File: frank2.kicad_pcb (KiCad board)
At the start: 2 copper layers, 77.3 x 99 mm, 150 parts, among them J1 USB Data, J2 Keyboard Data, Q1 BC850, Q2 BC850, SW1 Flash Button, SW2 Reset Button, SW3 Flash Button, U1 NCP1117-3.3_SOT223, U2 RP2040, Y1 ABM8-272-T3, Y2 ABM8-272-T3

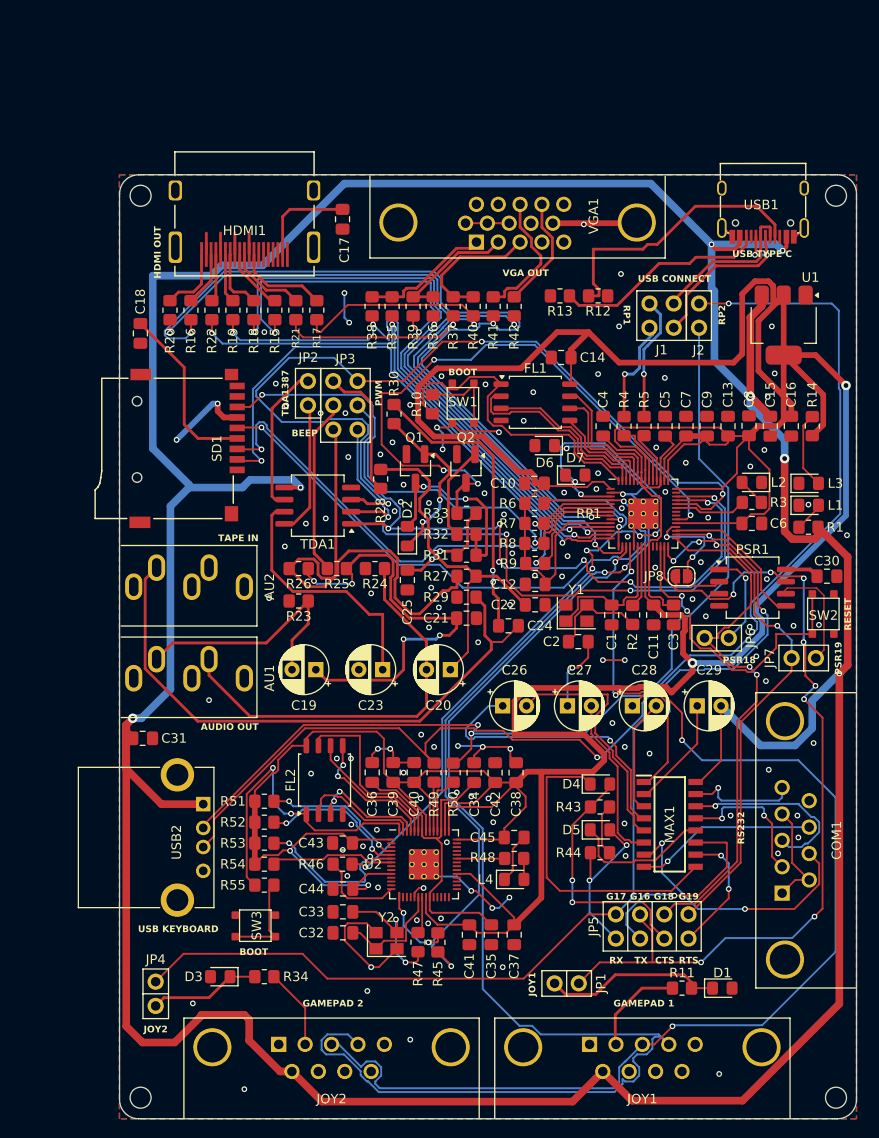
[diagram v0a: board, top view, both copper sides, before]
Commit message: Updated HW
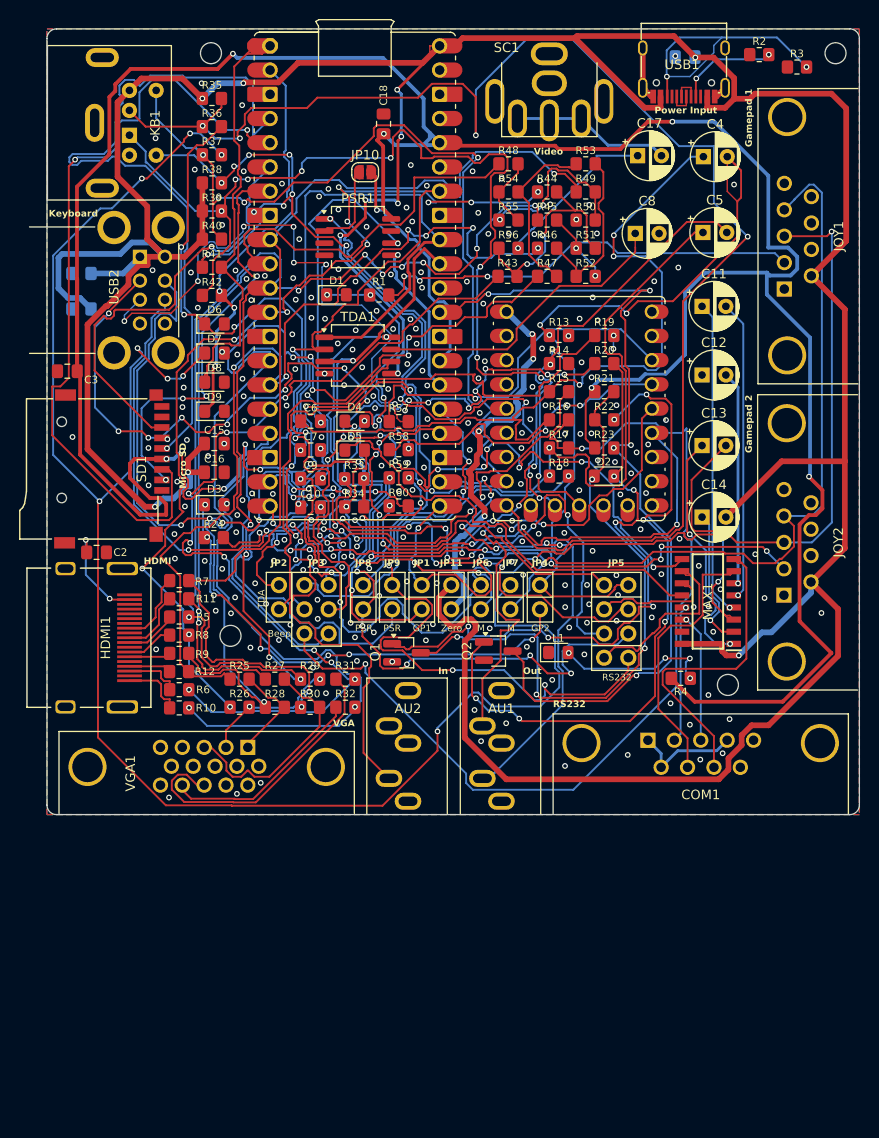
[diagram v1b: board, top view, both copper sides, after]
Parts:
- removed C21, C22: 10n, Capacitor_SMD:C_0805_2012Metric_Pad1.18x1.45mm_HandSolder
- removed C23: 10u, LIBS:Medved_CP_Radial_D5.0mm_P2.50mm
- removed C24, C25, C30: 0.1u, Capacitor_SMD:C_0805_2012Metric_Pad1.18x1.45mm_HandSolder
- removed C26, C27, C28, C29: 1u, LIBS:Medved_CP_Radial_D5.0mm_P2.50mm
- removed C31: 10u, Capacitor_SMD:C_0805_2012Metric_Pad1.18x1.45mm_HandSolder
- removed C32, C33: 15p, Capacitor_SMD:C_0805_2012Metric_Pad1.18x1.45mm_HandSolder
- removed C34, C35, C37, C39, C40, C41, C42, C43, C44, C45: 100n, Capacitor_SMD:C_0805_2012Metric_Pad1.18x1.45mm_HandSolder
- removed C36, C38: 1u, Capacitor_SMD:C_0805_2012Metric_Pad1.18x1.45mm_HandSolder
- removed FL1, FL2: W25Q128JVS, Package_SO:SOIC-8_5.23x5.23mm_P1.27mm
- removed J1: USB Data, LIBS:Medved_2x02
- removed J2: Keyboard Data, LIBS:Medved_PinHeader_1x02
- removed L2, L3, L4: LED, LED_SMD:LED_0805_2012Metric_Pad1.15x1.40mm_HandSolder
- removed REF** (x4): Medved_MountingHole_V2, LIBS:Medved_MountingHole_V2
- removed SW1, SW3: Flash Button, LIBS:Button_SMD_3x3x2
- removed SW2: Reset Button, LIBS:Button_SMD_3x3x2
- removed U1: NCP1117-3.3_SOT223, Package_TO_SOT_SMD:SOT-223-3_TabPin2
- removed U2: RP2040, LIBS:RP2040-QFN-56
- removed Y1, Y2: ABM8-272-T3, Crystal:Crystal_SMD_3225-4Pin_3.2x2.5mm
- added D8: 3V3, LIBS:Medved_D_0805, F.Cu at (94.8, 64.9)
- added D9: 3V3, LIBS:Medved_D_0805, F.Cu at (94.8, 67.9)
- added H1: MountingHole, LIBS:Medved_MountingHole_V2, F.Cu at (94.4, 30.4)
- added H2: MountingHole, LIBS:Medved_MountingHole_V2, F.Cu at (159.9, 30.4)
- added H3: MountingHole, LIBS:Medved_MountingHole_V2, F.Cu at (148.6, 96.6)
- added H4: MountingHole, LIBS:Medved_MountingHole_V2, F.Cu at (96.4, 91.5)
- added JP10: JMP PSRAM, Jumper:SolderJumper-2_P1.3mm_Open_RoundedPad1.0x1.5mm, F.Cu at (110.6, 42.8)
- added JP11: RP ZERO +5V Jumper, LIBS:Medved_PinHeader_1x02_P2.54mm_Vertical_R, F.Cu at (119.6, 86.1)
- added JP9: RP ZERO +5V Jumper, LIBS:Medved_PinHeader_1x02_P2.54mm_Vertical_R, F.Cu at (113.4, 86.1)
- added KB1: PS/2, LIBS:Connector_Mini-DIN_Female_6Pin_2rows, F.Cu at (85.8, 39.0)
- added R56: 51R*, LIBS:Medved_R_0805, F.Cu at (125.6, 50.8)
- added R57: 22R, LIBS:Medved_R_0805, F.Cu at (114.1, 69.0)
- added R58: 22R, LIBS:Medved_R_0805, F.Cu at (114.1, 71.9)
- added R59: 22R, LIBS:Medved_R_0805, F.Cu at (114.1, 74.9)
- added R60: 22R, LIBS:Medved_R_0805, F.Cu at (114.1, 77.8)
- added RP2: RP 2040 Zero, LIBS:rp2040-zero-tht, F.Cu at (133.0, 67.6)
- added SC1: VIDEO (Soft Composite), LIBS:AV_MOD_III-8.4-5, F.Cu at (129.9, 34.1)
- C1: value 15p -> 10u; footprint Capacitor_SMD:C_0805_2012Metric_Pad1.18x1.45mm_HandSolder -> LIBS:Medved_C_0805; moved to B.Cu
- C10, C3, C9: value 100n -> 0.1u; footprint Capacitor_SMD:C_0805_2012Metric_Pad1.18x1.45mm_HandSolder -> LIBS:Medved_C_0805
- C11, C12, C13, C14: value 100n -> 1u; footprint Capacitor_SMD:C_0805_2012Metric_Pad1.18x1.45mm_HandSolder -> LIBS:Medved_CP_Radial_D5.0mm_P2.50mm
- C15, C16: value 10u -> 0.1u; footprint Capacitor_SMD:C_0805_2012Metric_Pad1.18x1.45mm_HandSolder -> LIBS:Medved_C_0805
- C17: value 0.1u -> 220u; footprint Capacitor_SMD:C_0805_2012Metric_Pad1.18x1.45mm_HandSolder -> LIBS:Medved_CP_Radial_D5.0mm_P2.50mm
- C18: footprint Capacitor_SMD:C_0805_2012Metric_Pad1.18x1.45mm_HandSolder -> LIBS:Medved_C_0805
- C19, C20: footprint LIBS:Medved_CP_Radial_D5.0mm_P2.50mm -> LIBS:Medved_R_0805; moved to B.Cu
- C2: value 15p -> 0.1u; footprint Capacitor_SMD:C_0805_2012Metric_Pad1.18x1.45mm_HandSolder -> LIBS:Medved_C_0805
- C4, C8: value 100n -> 10u; footprint Capacitor_SMD:C_0805_2012Metric_Pad1.18x1.45mm_HandSolder -> LIBS:Medved_CP_Radial_D5.0mm_P2.50mm
- C5: value 1u -> 10u; footprint Capacitor_SMD:C_0805_2012Metric_Pad1.18x1.45mm_HandSolder -> LIBS:Medved_CP_Radial_D5.0mm_P2.50mm
- C6: value 100n -> 10n; footprint Capacitor_SMD:C_0805_2012Metric_Pad1.18x1.45mm_HandSolder -> LIBS:Medved_C_0805
- C7: value 1u -> 10n; footprint Capacitor_SMD:C_0805_2012Metric_Pad1.18x1.45mm_HandSolder -> LIBS:Medved_C_0805
- D1, D2, D3, D4, D5, D6, D7: footprint Diode_SMD:D_0805_2012Metric_Pad1.15x1.40mm_HandSolder -> LIBS:Medved_D_0805
- JP8: value JMP PSRAM -> RP ZERO +5V Jumper; footprint Jumper:SolderJumper-2_P1.3mm_Open_RoundedPad1.0x1.5mm -> LIBS:Medved_PinHeader_1x02_P2.54mm_Vertical_R
- L1: footprint LED_SMD:LED_0805_2012Metric_Pad1.15x1.40mm_HandSolder -> LIBS:Medved_L_0805
- R1: value 10K -> 1k; footprint Resistor_SMD:R_0805_2012Metric_Pad1.20x1.40mm_HandSolder -> LIBS:Medved_R_0805
- R10, R11, R47: value 1k -> 270R; footprint Resistor_SMD:R_0805_2012Metric_Pad1.20x1.40mm_HandSolder -> LIBS:Medved_R_0805
- R12: value 5.1K -> 270R; footprint Resistor_SMD:R_0805_2012Metric_Pad1.20x1.40mm_HandSolder -> LIBS:Medved_R_0805
- R13: value 5.1K -> 330R; footprint Resistor_SMD:R_0805_2012Metric_Pad1.20x1.40mm_HandSolder -> LIBS:Medved_R_0805
- R14: value 1K -> 330R; footprint Resistor_SMD:R_0805_2012Metric_Pad1.20x1.40mm_HandSolder -> LIBS:Medved_R_0805
- R15, R18: value 270R -> 1k; footprint Resistor_SMD:R_0805_2012Metric_Pad1.20x1.40mm_HandSolder -> LIBS:Medved_R_0805
- R16, R17: value 270R -> 2k; footprint Resistor_SMD:R_0805_2012Metric_Pad1.20x1.40mm_HandSolder -> LIBS:Medved_R_0805
- R19: value 270R -> 100R; footprint Resistor_SMD:R_0805_2012Metric_Pad1.20x1.40mm_HandSolder -> LIBS:Medved_R_0805
- R2: value 1k -> 5.1K; footprint Resistor_SMD:R_0805_2012Metric_Pad1.20x1.40mm_HandSolder -> LIBS:Medved_R_0805
- R20, R21, R22: value 270R -> 10k; footprint Resistor_SMD:R_0805_2012Metric_Pad1.20x1.40mm_HandSolder -> LIBS:Medved_R_0805
- R23, R24, R35: value 330R -> 1k; footprint Resistor_SMD:R_0805_2012Metric_Pad1.20x1.40mm_HandSolder -> LIBS:Medved_R_0805
- R25: value 1k -> 330R; footprint Resistor_SMD:R_0805_2012Metric_Pad1.20x1.40mm_HandSolder -> LIBS:Medved_R_0805
- R26, R27: value 2k -> 330R; footprint Resistor_SMD:R_0805_2012Metric_Pad1.20x1.40mm_HandSolder -> LIBS:Medved_R_0805
- R28, R38, R39, R40, R41, R42: footprint Resistor_SMD:R_0805_2012Metric_Pad1.20x1.40mm_HandSolder -> LIBS:Medved_R_0805
- R29: value 100R -> 1k; footprint Resistor_SMD:R_0805_2012Metric_Pad1.20x1.40mm_HandSolder -> LIBS:Medved_R_0805
- R3: value 1K -> 5.1K; footprint Resistor_SMD:R_0805_2012Metric_Pad1.20x1.40mm_HandSolder -> LIBS:Medved_R_0805
- R30: value 10k -> 1k; footprint Resistor_SMD:R_0805_2012Metric_Pad1.20x1.40mm_HandSolder -> LIBS:Medved_R_0805
- R31, R32: value 10k -> 100R; footprint Resistor_SMD:R_0805_2012Metric_Pad1.20x1.40mm_HandSolder -> LIBS:Medved_R_0805
- R33, R34: value 1k -> 1K; footprint Resistor_SMD:R_0805_2012Metric_Pad1.20x1.40mm_HandSolder -> LIBS:Medved_R_0805
- R36, R37: value 330R -> 100R; footprint Resistor_SMD:R_0805_2012Metric_Pad1.20x1.40mm_HandSolder -> LIBS:Medved_R_0805
- R4: value 27 -> 1K; footprint Resistor_SMD:R_0805_2012Metric_Pad1.20x1.40mm_HandSolder -> LIBS:Medved_R_0805
- R43: value 1K -> 750R*; footprint Resistor_SMD:R_0805_2012Metric_Pad1.20x1.40mm_HandSolder -> LIBS:Medved_R_0805
- R44, R48: value 1K -> 270R; footprint Resistor_SMD:R_0805_2012Metric_Pad1.20x1.40mm_HandSolder -> LIBS:Medved_R_0805
- R45, R46: value 100R -> 270R; footprint Resistor_SMD:R_0805_2012Metric_Pad1.20x1.40mm_HandSolder -> LIBS:Medved_R_0805
- R49, R5: value 27 -> 270R; footprint Resistor_SMD:R_0805_2012Metric_Pad1.20x1.40mm_HandSolder -> LIBS:Medved_R_0805
- R50: value 27 -> 300R; footprint Resistor_SMD:R_0805_2012Metric_Pad1.20x1.40mm_HandSolder -> LIBS:Medved_R_0805
- R51, R52, R53, R54: value 10K -> 150R; footprint Resistor_SMD:R_0805_2012Metric_Pad1.20x1.40mm_HandSolder -> LIBS:Medved_R_0805
- R55: value 1k -> 150R; footprint Resistor_SMD:R_0805_2012Metric_Pad1.20x1.40mm_HandSolder -> LIBS:Medved_R_0805
- R6, R7, R8, R9: value 10K -> 270R; footprint Resistor_SMD:R_0805_2012Metric_Pad1.20x1.40mm_HandSolder -> LIBS:Medved_R_0805
- RP1: value RP2040 -> RP2040 Pico; footprint LIBS:RP2040-QFN-56 -> LIBS:Raspberry_Pi_Pico_SMT_THT_MOD_2
- USB2: value USB_A -> USB_A_Stacked; footprint LIBS:Medved_USB_A -> LIBS:Medved_USB_A_CUI_UJ2-ADH-TH_Horizontal_Stacked
- moved D1 83.2 mm to (107.6, 55.7)
- moved JOY1 81.8 mm to (154.5, 55.1), turned to 90 degrees
- moved R53 78.8 mm to (133.7, 42.0), turned to 0 degrees
- moved R45 76.6 mm to (129.7, 47.9), turned to 0 degrees
- moved R54 75.0 mm to (125.6, 44.9), turned to 0 degrees
- moved R55 74.3 mm to (125.6, 47.9)
- moved R48 72.9 mm to (125.6, 42.0), turned to 0 degrees
- moved R47 71.1 mm to (129.7, 53.8), turned to 0 degrees
- moved JOY2 70.9 mm to (154.5, 87.2), turned to 90 degrees
- moved R44 69.5 mm to (129.7, 44.9)
- moved C3 68.5 mm to (79.3, 63.7), turned to 0 degrees
- moved R46 68.1 mm to (129.7, 50.8)
- moved R51 67.1 mm to (133.7, 50.8), turned to 0 degrees
- moved R11 66.7 mm to (91.1, 87.6), turned to 0 degrees
- moved R52 66.4 mm to (133.7, 53.8), turned to 0 degrees
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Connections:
- net /PW_D+ renamed /Power/D+
- net /PW_D- renamed /Power/D-
- net /RP2040/GPIO23 renamed /Pico/GPIO29_1
- C1 pad 1: /RP2040/XIN -> VBUS
- C11 pad 1: +3V3 -> /RS232/C2+
- C11 pad 2: GND -> /RS232/C2-
- C12 pad 1: +3V3 -> GND
- C12 pad 2: GND -> /RS232/V-
- C13 pad 1: +3V3 -> /RS232/C1+
- C13 pad 2: GND -> /RS232/C1-
- C14 pad 1: +3V3 -> /RS232/V+
- C14 pad 2: GND -> VBUS
- C16 pad 1: +3V3 -> VBUS
- C17 pad 1: /HDMI/VBUS -> Net-(C17-Pad1)
- C17 pad 2: GND -> /Composite Video/CVBS
- C18 pad 1: GND -> +3V3
- C18 pad 2: /SD/+3V3 -> GND
- C19 pad 1: Net-(C19-Pad1) -> VBUS
- C19 pad 2: /Audio/L -> GND
- C2 pad 1: Net-(C2-Pad1) -> /HDMI/VBUS
- C20 pad 1: Net-(C20-Pad1) -> VBUS
- C20 pad 2: /Audio/R -> GND
- C3 pad 1: Net-(RP1-VREG_VOUT) -> GND
- C3 pad 2: GND -> +3V3
- C4 pad 1: Net-(RP1-VREG_VOUT) -> Net-(C4-Pad1)
- C4 pad 2: GND -> /Audio/L
- C5 pad 1: Net-(RP1-VREG_VOUT) -> Net-(C5-Pad1)
- C5 pad 2: GND -> /Audio/R
- C6 pad 1: +3V3 -> Net-(C4-Pad1)
- C7 pad 1: +3V3 -> Net-(C5-Pad1)
- C8 pad 1: +3V3 -> /Audio/FLT
- C9 pad 1: +3V3 -> /Audio/LOAD_IN
- C9 pad 2: GND -> Net-(C9-Pad2)
- D6 pad 1: /GPIO0 -> Net-(D6-K)
- D7 pad 1: /GPIO1 -> Net-(D7-K)
- JP6 pad 1: Net-(JP6-A) -> /GPIO15
- JP6 pad 2: /GPIO18 -> Net-(D6-K)
- JP7 pad 1: /GPIO19 -> Net-(D7-K)
- JP7 pad 2: Net-(JP7-B) -> /GPIO14
- JP8 pad 2: /GPIO21 -> /GPIO18
- PSR1 pad 1: Net-(JP6-A) -> Net-(JP8-A)
- PSR1 pad 2: Net-(JP8-A) -> Net-(JP10-A)
- PSR1 pad 6: Net-(JP7-B) -> Net-(JP9-B)
- PSR1 pad 8: /PSRAM/+3V3 -> +3V3
- R1 pad 1: Net-(L1-A) -> Net-(D1-K)
- R1 pad 2: VBUS -> /Gamepad 1/J2_DATA
- R10 pad 1: /RP2040/QSPI_SS -> /HDMI/D2P
- R10 pad 2: /RP2040/~{USB_BOOT} -> /GPIO13
- R11 pad 1: Net-(D1-K) -> /HDMI/CLKP
- R11 pad 2: /Gamepad 1/J2_DATA -> /GPIO7
- R12 pad 1: GND -> /HDMI/D1P
- R12 pad 2: Net-(USB1-CC1) -> /GPIO11
- R13 pad 1: GND -> /Audio/L
- R13 pad 2: Net-(USB1-CC2) -> GND
- R14 pad 1: Net-(L3-A) -> /Audio/R
- R14 pad 2: +3V3 -> GND
- R15 pad 1: /HDMI/D0N -> Net-(C4-Pad1)
- R15 pad 2: /GPIO8 -> /Audio/LEFT_OUT
- R16 pad 1: /HDMI/D2N -> Net-(C4-Pad1)
- R16 pad 2: /GPIO12 -> /Audio/BEEP_OUT
- R17 pad 1: /HDMI/CLKN -> Net-(C5-Pad1)
- R17 pad 2: /GPIO6 -> /Audio/BEEP_OUT
- R18 pad 1: /HDMI/D0P -> Net-(C5-Pad1)
- R18 pad 2: /GPIO9 -> /Audio/RIGHT_OUT
- R19 pad 1: /HDMI/D1N -> /Audio/LOAD_IN
- R19 pad 2: /GPIO10 -> GND
- R2 pad 1: /RP2040/XOUT -> GND
- R2 pad 2: Net-(C2-Pad1) -> Net-(USB1-CC1)
- R20 pad 1: /HDMI/D2P -> Net-(C9-Pad2)
- R20 pad 2: /GPIO13 -> Net-(D2-K)
- R21 pad 1: /HDMI/CLKP -> +3V3
- R21 pad 2: /GPIO7 -> Net-(D2-A)
- R22 pad 1: /HDMI/D1P -> Net-(D2-A)
- R22 pad 2: /GPIO11 -> Net-(Q2-B)
- R23 pad 1: /Audio/L -> +3V3
- R23 pad 2: GND -> /GPIO22
- R24 pad 1: /Audio/R -> Net-(D3-K)
- R24 pad 2: GND -> /Gamepad 2/J2_DATA
- R25 pad 1: Net-(C19-Pad1) -> /GPIO11
- R25 pad 2: /Audio/LEFT_OUT -> /VGA/VGA_RH
- R26 pad 1: Net-(C19-Pad1) -> /GPIO9
- R26 pad 2: /Audio/BEEP_OUT -> /VGA/VGA_GH
- R27 pad 1: Net-(C20-Pad1) -> /GPIO7
- R27 pad 2: /Audio/BEEP_OUT -> /VGA/VGA_BH
- R28 pad 1: Net-(C20-Pad1) -> /GPIO10
- R28 pad 2: /Audio/RIGHT_OUT -> /VGA/VGA_RH
- R29 pad 1: /Audio/LOAD_IN -> /GPIO8
- R29 pad 2: GND -> /VGA/VGA_GH
- R3 pad 1: Net-(L2-A) -> GND
- R3 pad 2: /RP2040/GPIO25 -> Net-(USB1-CC2)
- R30 pad 1: Net-(C24-Pad2) -> /GPIO6
- R30 pad 2: Net-(D2-K) -> /VGA/VGA_BH
- R31 pad 1: /Audio/+3V3 -> /VGA/VGA_HS
- R31 pad 2: Net-(D2-A) -> /GPIO12
- R32 pad 1: Net-(D2-A) -> /VGA/VGA_VS
- R32 pad 2: Net-(Q2-B) -> /GPIO13
- R33 pad 1: /Audio/+3V3 -> /RS232/CTS_PICO
- R33 pad 2: /GPIO22 -> +3V3
- R34 pad 1: Net-(D3-K) -> /RS232/RX_PICO
- R34 pad 2: /Gamepad 2/J2_DATA -> +3V3
- R35 pad 1: /GPIO11 -> VBUS
- R35 pad 2: /VGA/VGA_RH -> /ZGPIO14
- R36 pad 1: /GPIO9 -> /ZGPIO14
- R36 pad 2: /VGA/VGA_GH -> Net-(D6-K)
- R37 pad 1: /GPIO7 -> /ZGPIO15
- R37 pad 2: /VGA/VGA_BH -> Net-(D7-K)
- R38 pad 1: /GPIO10 -> VBUS
- R38 pad 2: /VGA/VGA_RH -> /ZGPIO12
- R39 pad 1: /GPIO8 -> VBUS
- R39 pad 2: /VGA/VGA_GH -> /ZGPIO11
- R4 pad 1: /D+ -> Net-(L1-A)
- R4 pad 2: Net-(RP1-USB_DP) -> +3V3
- R40 pad 1: /GPIO6 -> VBUS
- R40 pad 2: /VGA/VGA_BH -> /ZGPIO15
- R41 pad 1: /VGA/VGA_HS -> /ZGPIO12
- R41 pad 2: /GPIO12 -> /GPIO0
- R42 pad 1: /VGA/VGA_VS -> /ZGPIO11
- R42 pad 2: /GPIO13 -> /GPIO1
- R43 pad 1: /RS232/CTS_PICO -> /GPIO12
- R43 pad 2: /RS232/+3V3 -> Net-(R43-Pad2)
- R44 pad 1: /RS232/RX_PICO -> /GPIO9
- R44 pad 2: /RS232/+3V3 -> Net-(R43-Pad2)
- R45 pad 1: /Keyboard/GPIO12 -> /GPIO8
- R45 pad 2: /GPIO0 -> Net-(R45-Pad2)
- R46 pad 1: /Keyboard/GPIO11 -> /GPIO11
- R46 pad 2: /GPIO1 -> Net-(R46-Pad2)
- R47 pad 1: /Keyboard/RP2040/XOUT -> /GPIO10
- R47 pad 2: Net-(C33-Pad1) -> Net-(R47-Pad2)
- R48 pad 1: Net-(L4-A) -> /GPIO7
- R48 pad 2: /Keyboard/RP2040/GPIO25 -> Net-(R48-Pad2)
- R49 pad 1: /KB_D+ -> /GPIO6
- R49 pad 2: Net-(U2-USB_DP) -> Net-(R49-Pad2)
- R5 pad 1: /D- -> /HDMI/D0N
- R5 pad 2: Net-(RP1-USB_DM) -> /GPIO8
- R50 pad 1: /KB_D- -> GND
- R50 pad 2: Net-(U2-USB_DM) -> Net-(R49-Pad2)
- R51 pad 1: /Keyboard/RP2040/GPIO2 -> Net-(R45-Pad2)
- R51 pad 2: +3V3 -> Net-(R43-Pad2)
- R52 pad 1: /Keyboard/RP2040/GPIO3 -> Net-(R46-Pad2)
- R52 pad 2: +3V3 -> Net-(R45-Pad2)
- R53 pad 1: /Keyboard/RP2040/GPIO4 -> Net-(R47-Pad2)
- R53 pad 2: +3V3 -> Net-(R46-Pad2)
- R54 pad 1: /Keyboard/RP2040/GPIO5 -> Net-(R48-Pad2)
- R54 pad 2: +3V3 -> Net-(R47-Pad2)
- R55 pad 1: /Keyboard/RP2040/QSPI_SS -> Net-(R49-Pad2)
- R55 pad 2: /Keyboard/RP2040/~{USB_BOOT} -> Net-(R48-Pad2)
- R6 pad 1: /GPIO2 -> /HDMI/D2N
- R6 pad 2: +3V3 -> /GPIO12
- R7 pad 1: /GPIO3 -> /HDMI/CLKN
- R7 pad 2: +3V3 -> /GPIO6
- R8 pad 1: /GPIO4 -> /HDMI/D0P
- R8 pad 2: +3V3 -> /GPIO9
- R9 pad 1: /GPIO5 -> /HDMI/D1N
- R9 pad 2: +3V3 -> /GPIO10
- RP1 pad 1: +3V3 -> /GPIO0
- RP1 pad 10: +3V3 -> /GPIO7
- RP1 pad 13: /GPIO10 -> GND
- RP1 pad 14: /GPIO11 -> /GPIO10
- RP1 pad 15: /GPIO12 -> /GPIO11
- RP1 pad 16: /GPIO13 -> /GPIO12
- RP1 pad 17: /GPIO14 -> /GPIO13
- RP1 pad 18: /GPIO15 -> GND
- RP1 pad 19: GND -> /GPIO14
- RP1 pad 2: /GPIO0 -> /GPIO1
- RP1 pad 20: /RP2040/XIN -> /GPIO15
- RP1 pad 21: /RP2040/XOUT -> /GPIO16
- RP1 pad 22: +3V3 -> /GPIO17
- RP1 pad 23: Net-(RP1-VREG_VOUT) -> GND
- RP1 pad 24: /RP2040/SWCLK -> /GPIO18
- RP1 pad 25: /RP2040/SWD -> /GPIO19
- RP1 pad 26: /RUN -> /GPIO20
- RP1 pad 27: /GPIO16 -> /GPIO21
- RP1 pad 28: /GPIO17 -> GND
- RP1 pad 29: /GPIO18 -> /GPIO22
- RP1 pad 3: /GPIO1 -> GND
- RP1 pad 30: /GPIO19 -> /Pico/RUN
- RP1 pad 31: /GPIO20 -> /GPIO26
- RP1 pad 32: /GPIO21 -> /GPIO27
- RP1 pad 33: +3V3 -> GND
- RP1 pad 34: /GPIO22 -> /GPIO28
- RP1 pad 36: /RP2040/GPIO24 -> +3V3
- RP1 pad 37: /RP2040/GPIO25 -> /Pico/3V3_IN
- RP1 pad 38: /GPIO26 -> GND
- RP1 pad 39: /GPIO27 -> /Pico/VBUS_IN
- RP1 pad 40: /GPIO28 -> VBUS
- RP1 pad 8: /GPIO6 -> GND
- RP1 pad 9: /GPIO7 -> /GPIO6
- SD1 pad 4: /SD/+3V3 -> +3V3
- USB2 pad 2: /KB_D- -> Net-(USB2-D1-)
- USB2 pad 3: /KB_D+ -> Net-(USB2-D1+)
- USB2 pad 5: GND -> VBUS
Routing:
- net Net-(D7-K): track 0.00 -> 181.0 mm, vias 0 -> 8
- net +3V3: track 494.1 -> 323.8 mm, vias 4 -> 14
- net /ZGPIO14: track 0.00 -> 153.1 mm, vias 0 -> 4
- net /KB_D+: track 130.1 -> 0.00 mm, vias 2 -> 0
- net /ZGPIO11: track 0.00 -> 113.0 mm, vias 0 -> 9
- net /KB_D-: track 102.5 -> 0.00 mm, vias 2 -> 0
- net GND: track 116.9 -> 21.8 mm, vias 125 -> 229
- net /ZGPIO15: track 0.00 -> 94.7 mm, vias 0 -> 4
- net /ZGPIO12: track 0.00 -> 94.5 mm, vias 0 -> 12
- net Net-(C5-Pad1): track 0.00 -> 92.6 mm, vias 0 -> 7
- net Net-(D6-K): track 0.00 -> 91.8 mm, vias 0 -> 10
- net /GPIO8: track 67.1 -> 149.0 mm, vias 3 -> 12
- net Net-(C4-Pad1): track 0.00 -> 81.5 mm, vias 0 -> 3
- net Net-(JP9-B): track 0.00 -> 81.4 mm, vias 0 -> 1
- net /GPIO17: track 114.3 -> 39.9 mm, vias 3 -> 6
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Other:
- board size 77.3 x 99 mm -> 85.2 x 82.4 mm
- board text added: "Beep"
- board text added: "GP1"
- board text added: "GP2"
- board text added: "Gamepad 1"
- board text added: "Gamepad 2"
- board text added: "HDMI"
- board text added: "In"
- board text added: "Keyboard"
- board text added: "M"
- board text added: "Micro SD"
- board text added: "Out"
- board text added: "PSR"
- board text added: "Power Input"
- board text added: "TDA"
- board text added: "VGA"
- board text added: "Video"
- board text added: "Zero"
- board text removed: "AUDIO OUT"
- board text removed: "BEEP"
- board text removed: "BOOT"
- board text removed: "CTS"
- board text removed: "G16"
- board text removed: "G17"
- board text removed: "G18"
- board text removed: "G19"
- board text removed: "GAMEPAD 1"
- board text removed: "GAMEPAD 2"
- board text removed: "HDMI OUT"
- board text removed: "JOY1"
- board text removed: "JOY2"
- board text removed: "PSR18"
- board text removed: "PSR19"
- board text removed: "PWM"
- board text removed: "RESET"
- board text removed: "RP1"
- board text removed: "RP2"
- board text removed: "RTS"
- board text removed: "RX"
- board text removed: "TAPE IN"
- board text removed: "TDA1387"
- board text removed: "TX"
- board text removed: "USB CONNECT"
- board text removed: "USB KEYBOARD"
- board text removed: "USB TYPE C"
- board text removed: "VGA OUT"
